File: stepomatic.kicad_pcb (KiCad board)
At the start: 2 copper layers, 50 x 30 mm, 80 parts, among them J1 I2C, J2 Conn_01x03, J4 USB_B_Micro, Q1 MMBT3904, Q2 MMBT3904, SW1 Mode, SW2 RST, U1 HDC1080DMBR, U3 ULN2003A, U4 CH340C, U5 28BYJ-48, U6 AMS1117, U7 ESP-07

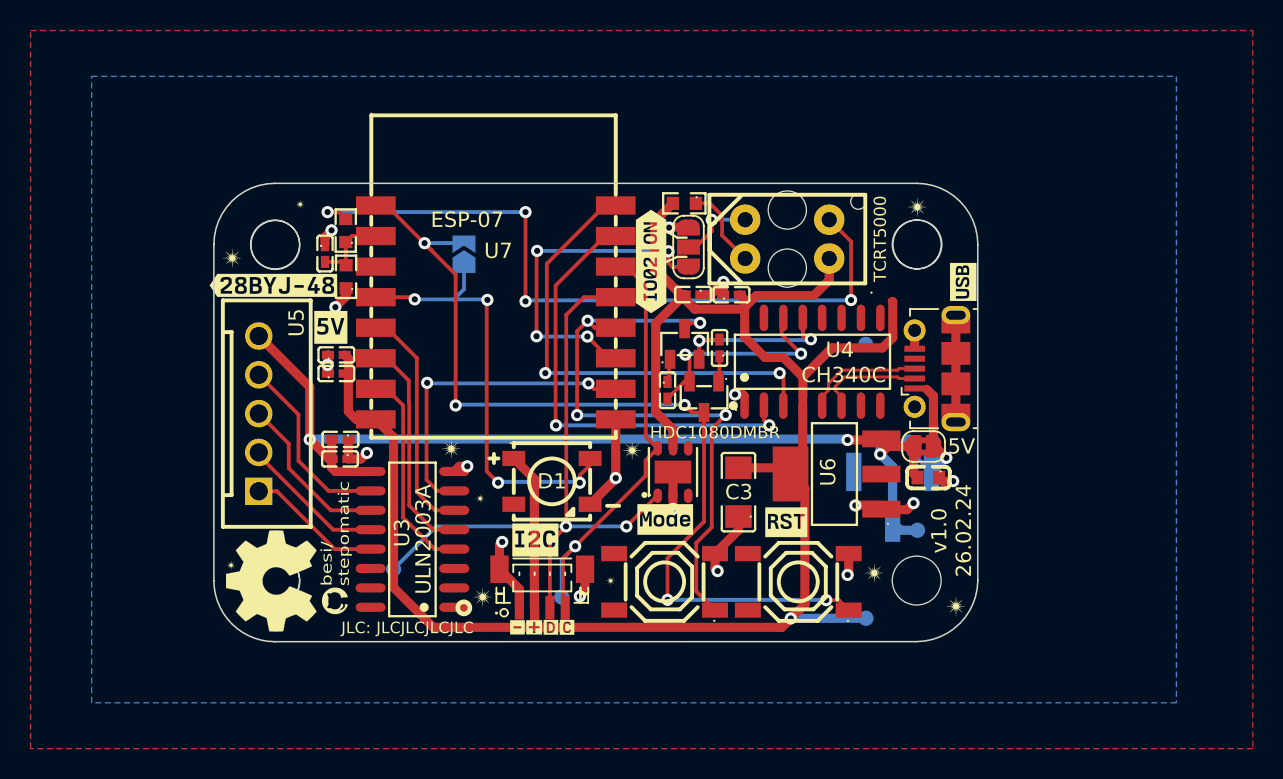
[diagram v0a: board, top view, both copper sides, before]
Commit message: Finish up PCB backside artwork
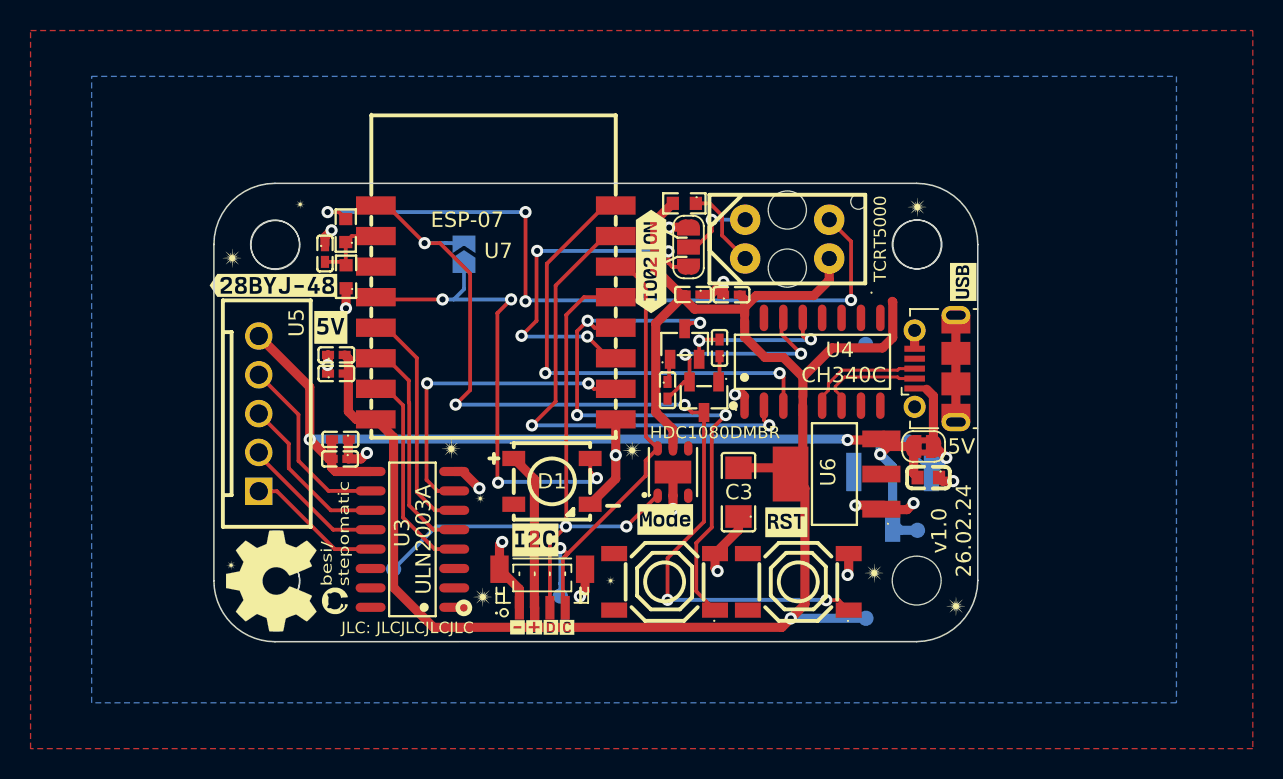
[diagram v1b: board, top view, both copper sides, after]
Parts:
- added G***: LOGO, LOGO, B.Cu at (110.3, 72.8)
- added G***: LOGO, LOGO, B.Cu at (116.7, 80.2)
- added G***: LOGO, LOGO, B.Cu at (113.1, 77.8)
- J2: value Conn_01x03 -> 5V Switch
- moved G*** 1.89 mm to (109.8, 72.2)
- moved G*** 1.33 mm to (112.9, 81.8)
- moved TP1 0.11 mm to (122.7, 97.0)
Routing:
- net NEOPIXEL: track 29.0 -> 31.5 mm
- net RX: track 30.4 -> 32.6 mm
- net IR: track 22.2 -> 23.5 mm
- net RESET: track 60.8 -> 62.2 mm
- net GND: track 47.8 -> 48.7 mm
- net I2C_SCL: track 30.2 -> 30.7 mm
